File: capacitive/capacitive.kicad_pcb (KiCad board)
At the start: 2 copper layers, 64 x 77 mm, 63 parts, among them J101 UL, J102 UART, J103 SWD, J104 TX_PADS, J105 RX_PAD, J106 POWER, J107 UR, J108 LL, J109 LR, Q101 RU1C002ZPTCL, SW101 SW_Push, U101 STM32F070C6T6, U102 TLV9062IDR, U103 SG7050CAN_8.000000M-TJGA3, U104 TLV74133PDBVR

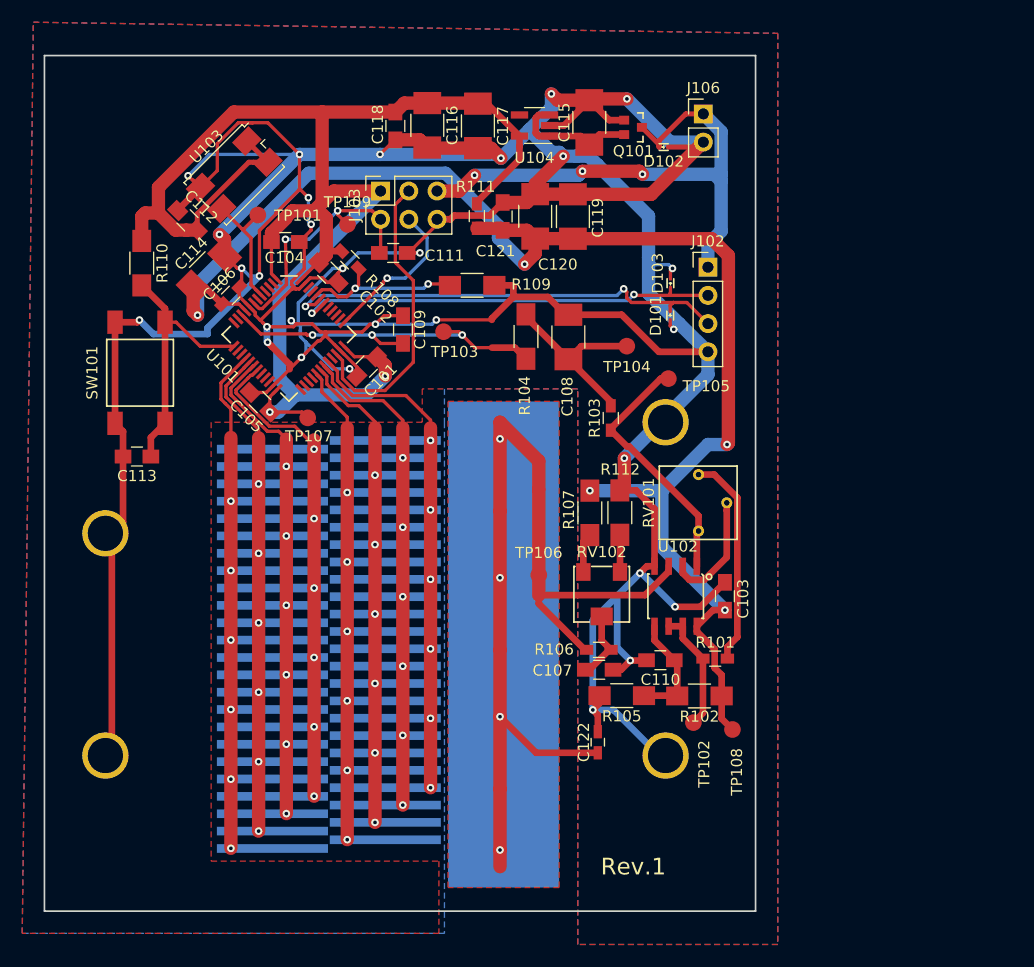
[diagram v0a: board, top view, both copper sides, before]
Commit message: Change scale size and finish relayout
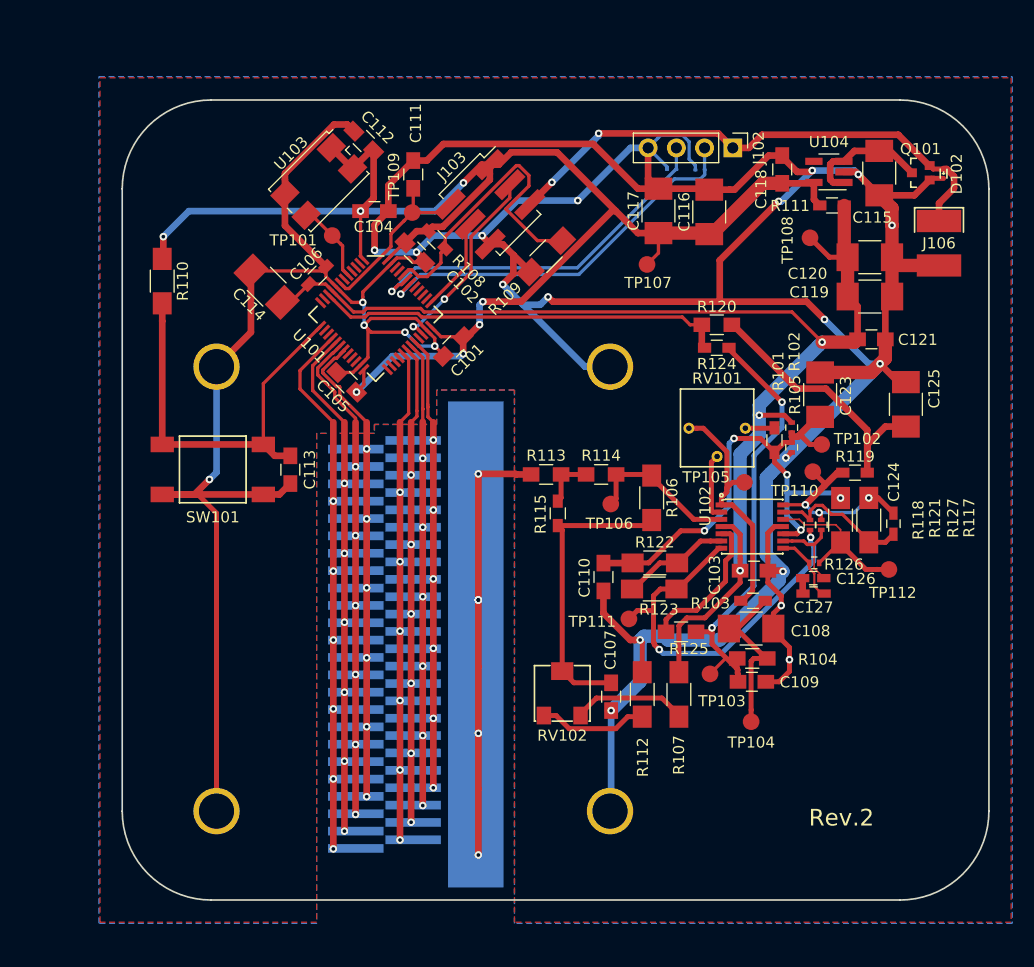
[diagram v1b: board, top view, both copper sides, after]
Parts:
- removed C122: 16pF 5%, Capacitors_SMD:C_0603_HandSoldering
- added C123: 10uF 10%, Capacitors_SMD:C_1210_HandSoldering, F.Cu at (133.8, 82.5)
- added C124: 1.8nF 2%, Capacitors_SMD:C_0603_HandSoldering, F.Cu at (140.4, 94.1)
- added C125: 100nF 2%, Capacitors_SMD:C_1210_HandSoldering, F.Cu at (141.5, 83.4)
- added C126: 33nF 5%, Capacitors_SMD:C_0603_HandSoldering, F.Cu at (133.2, 99.0)
- added C127: 33nF 5%, Capacitors_SMD:C_0603_HandSoldering, F.Cu at (133.2, 100.4)
- added R113: 0, Resistors_SMD:R_0805_HandSoldering, F.Cu at (109.2, 89.7)
- added R114: 0, Resistors_SMD:R_0805_HandSoldering, F.Cu at (114.1, 89.7)
- added R115: DNP, Resistors_SMD:R_0603_HandSoldering, F.Cu at (110.2, 93.2)
- added R117: 100k 1%, Resistors_SMD:R_1206_HandSoldering, F.Cu at (138.2, 93.8)
- added R118: 10k 1%, Resistors_SMD:R_0402, F.Cu at (132.9, 94.2)
- added R119: 1.58k 1%, Resistors_SMD:R_0603_HandSoldering, F.Cu at (136.9, 89.5)
- added R120: 0, Resistors_SMD:R_0805_HandSoldering, F.Cu at (124.5, 76.2)
- added R121: 10k 1%, Resistors_SMD:R_0402, F.Cu at (133.9, 94.2)
- added R122: 100k 1%, Resistors_SMD:R_1206_HandSoldering, F.Cu at (118.9, 97.7)
- added R123: 100k 1%, Resistors_SMD:R_1206_HandSoldering, F.Cu at (118.9, 100.0)
- added R124: DNP, Resistors_SMD:R_0603_HandSoldering, F.Cu at (124.5, 78.3)
- added R125: 0, Resistors_SMD:R_0805_HandSoldering, F.Cu at (121.3, 103.9)
- added R126: 1k 1%, Resistors_SMD:R_0402, F.Cu at (133.3, 97.7)
- added R127: 100k 1%, Resistors_SMD:R_1206_HandSoldering, F.Cu at (135.7, 93.8)
- added TP110: TEST, Measurement_Points:Measurement_Point_Round-SMD-Pad_Small, F.Cu at (133.2, 89.5)
- added TP111: TEST, Measurement_Points:Measurement_Point_Round-SMD-Pad_Small, F.Cu at (116.6, 102.7)
- added TP112: TEST, Measurement_Points:Measurement_Point_Round-SMD-Pad_Small, F.Cu at (140.0, 98.2)
- C109: value 10nF 1% -> 10 nF 1%
- D101, D103: moved to B.Cu
- J103: footprint Socket_Strips:Socket_Strip_Straight_2x03_Pitch2.54mm -> Socket_Strips:Socket_Strip_Straight_2x03_Pitch2.54mm_SMD
- J106: footprint Socket_Strips:Socket_Strip_Straight_1x02_Pitch2.54mm -> capacitive:Power_Pads
- R101: value 100 1% -> 1k
- R102, R105: value 100k 1% -> 1k 1%; footprint Resistors_SMD:R_1206_HandSoldering -> Resistors_SMD:R_0402
- R104: footprint Resistors_SMD:R_1206_HandSoldering -> Resistors_SMD:R_0805_HandSoldering
- R106: value 10M 5% -> 100k 1%; footprint Resistors_SMD:R_0603_HandSoldering -> Resistors_SMD:R_1206_HandSoldering
- U102: value TLV9062IDR -> TLV9064IPWR; footprint capacitive:TI_SOIC-8 -> capacitive:TI_TSSOP14
- moved TP108 44.8 mm to (132.9, 68.4)
- moved C109 44.6 mm to (127.7, 108.4), turned to 0 degrees
- moved TP103 39.0 mm to (123.9, 107.7)
- moved TP104 35.6 mm to (127.6, 112.0)
- moved R104 35.4 mm to (127.7, 106.3), turned to 180 degrees
- moved C118 35.0 mm to (130.4, 62.2), turned to 90 degrees
- moved J101 35.0 mm to (100.0, 80.0)
- moved C121 35.0 mm to (138.4, 77.5), turned to 0 degrees
- moved TP107 33.5 mm to (118.2, 70.8)
- moved R111 32.0 mm to (134.9, 65.5), turned to 0 degrees
- moved C108 31.0 mm to (127.6, 103.6), turned to 0 degrees
- moved C120 30.3 mm to (138.3, 70.2), turned to 0 degrees
- moved C119 27.7 mm to (138.3, 73.7), turned to 0 degrees
- moved TP102 27.6 mm to (133.9, 87.0), turned to 0 degrees
- moved R105 27.1 mm to (131.2, 87.3), turned to 270 degrees
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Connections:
- C109 pad 1: /ADC_IN -> /A
- C110 pad 1: Net-(C110-Pad1) -> /+1V65
- Q101 pad 2: Net-(C115-Pad1) -> +5V
- Q101 pad 3: +5V -> Net-(C115-Pad1)
- R102 pad 2: Net-(C110-Pad1) -> /+1V65
- R104 pad 2: /ADC_IN -> /A
- R105 pad 1: Net-(C110-Pad1) -> /+1V65
- R106 pad 1: /RX_PAD -> Net-(R106-Pad1)
- TP103 pad 1: /ADC_IN -> /A
- TP106 pad 1: /RX_PAD -> Net-(R106-Pad1)
- U102 pad 3: /RX_PAD -> Net-(R106-Pad1)
- U102 pad 4: GND -> +3.3VA
- U102 pad 5: Net-(C110-Pad1) -> Net-(R125-Pad2)
- U102 pad 6: /+1V65 -> Net-(R122-Pad2)
- U102 pad 7: /+1V65 -> Net-(R118-Pad1)
- U102 pad 8: +3.3VA -> Net-(C127-Pad1)
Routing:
- net /RX_PAD: track 88.8 -> 39.1 mm, vias 4 -> 5
- net /A: track 0.00 -> 41.7 mm, vias 0 -> 2
- net /+1V65: track 11.1 -> 47.2 mm, vias 0 -> 5
- net Net-(R118-Pad1): track 0.00 -> 35.9 mm, vias 0 -> 2
- net GND: track 455.3 -> 426.2 mm, vias 29 -> 23
- net Net-(C125-Pad1): track 0.00 -> 24.8 mm
- net Net-(C107-Pad1): track 6.41 -> 26.8 mm
- net Net-(C124-Pad2): track 0.00 -> 18.3 mm, vias 0 -> 3
- net +3.3VA: track 133.0 -> 116.1 mm, vias 5 -> 3
- net Net-(R101-Pad2): track 19.2 -> 2.63 mm
- net Net-(R126-Pad1): track 0.00 -> 14.8 mm
- net Net-(R106-Pad1): track 0.00 -> 14.1 mm
- net /ZERO: track 23.9 -> 37.4 mm
- net Net-(R125-Pad2): track 0.00 -> 13.2 mm
- net Net-(C124-Pad1): track 0.00 -> 13.0 mm
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- removed copper zone on F.Cu, net /RX_PAD
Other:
- board size 64 x 77 mm -> 78 x 72 mm
- board text added: "Rev.2"
- board text removed: "Rev.1"
